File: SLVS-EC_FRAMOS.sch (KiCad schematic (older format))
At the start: 10 parts, among them J21 DF40HC(4.0)-60DS-0.4V(51)

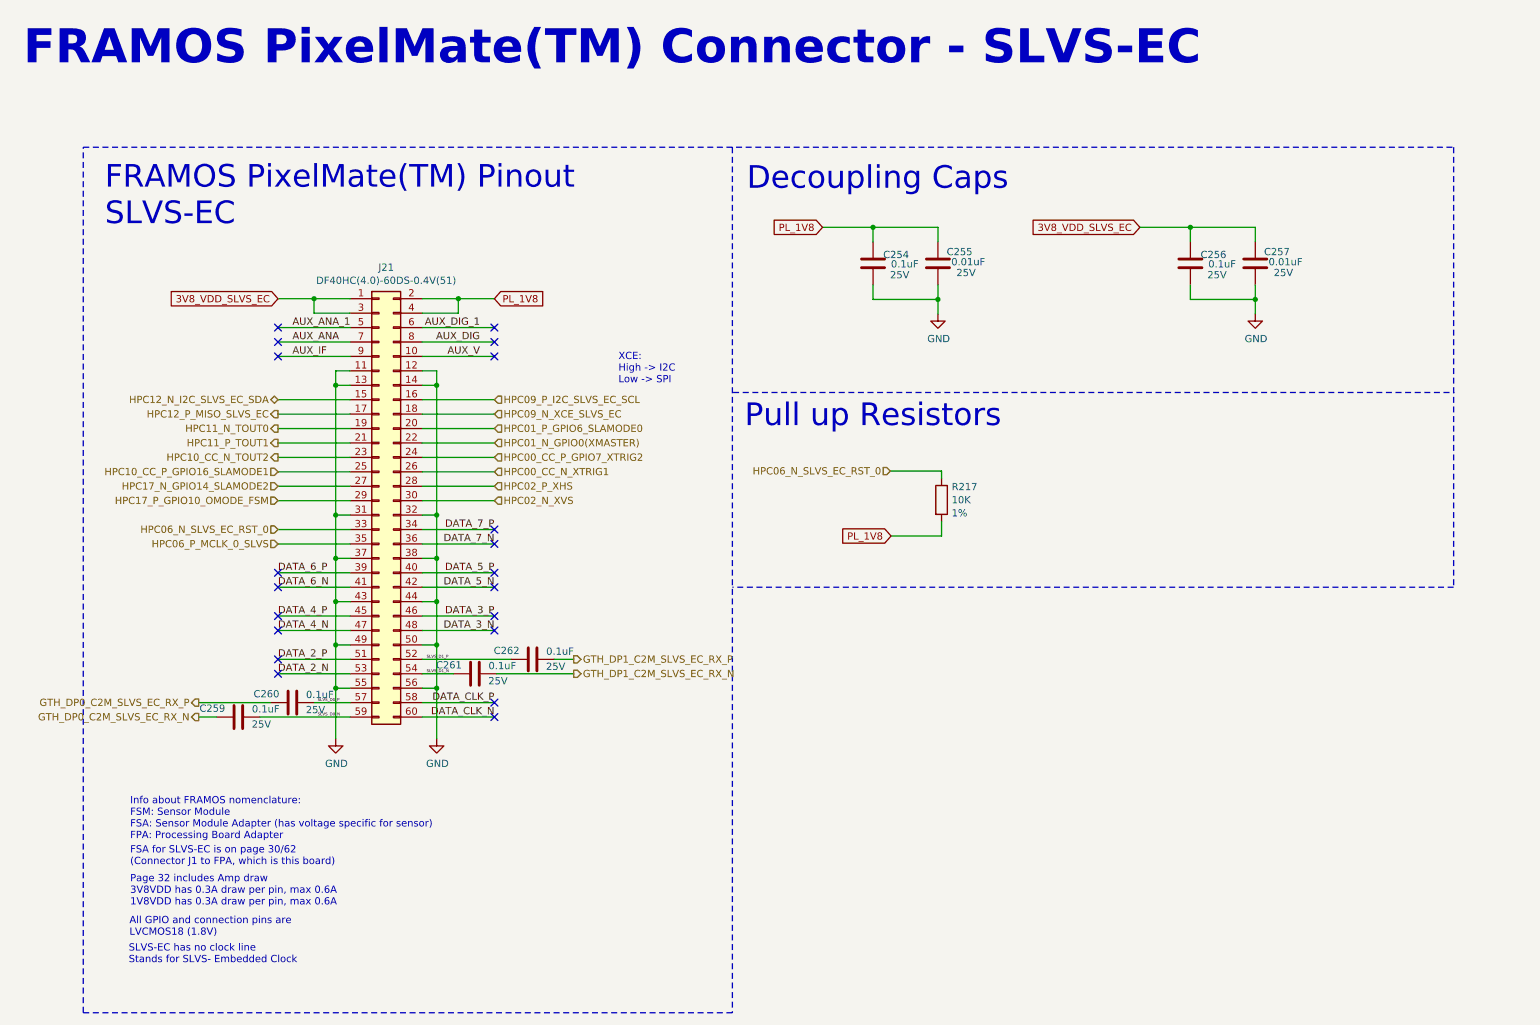
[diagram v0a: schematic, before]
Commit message: Pre-Production Push
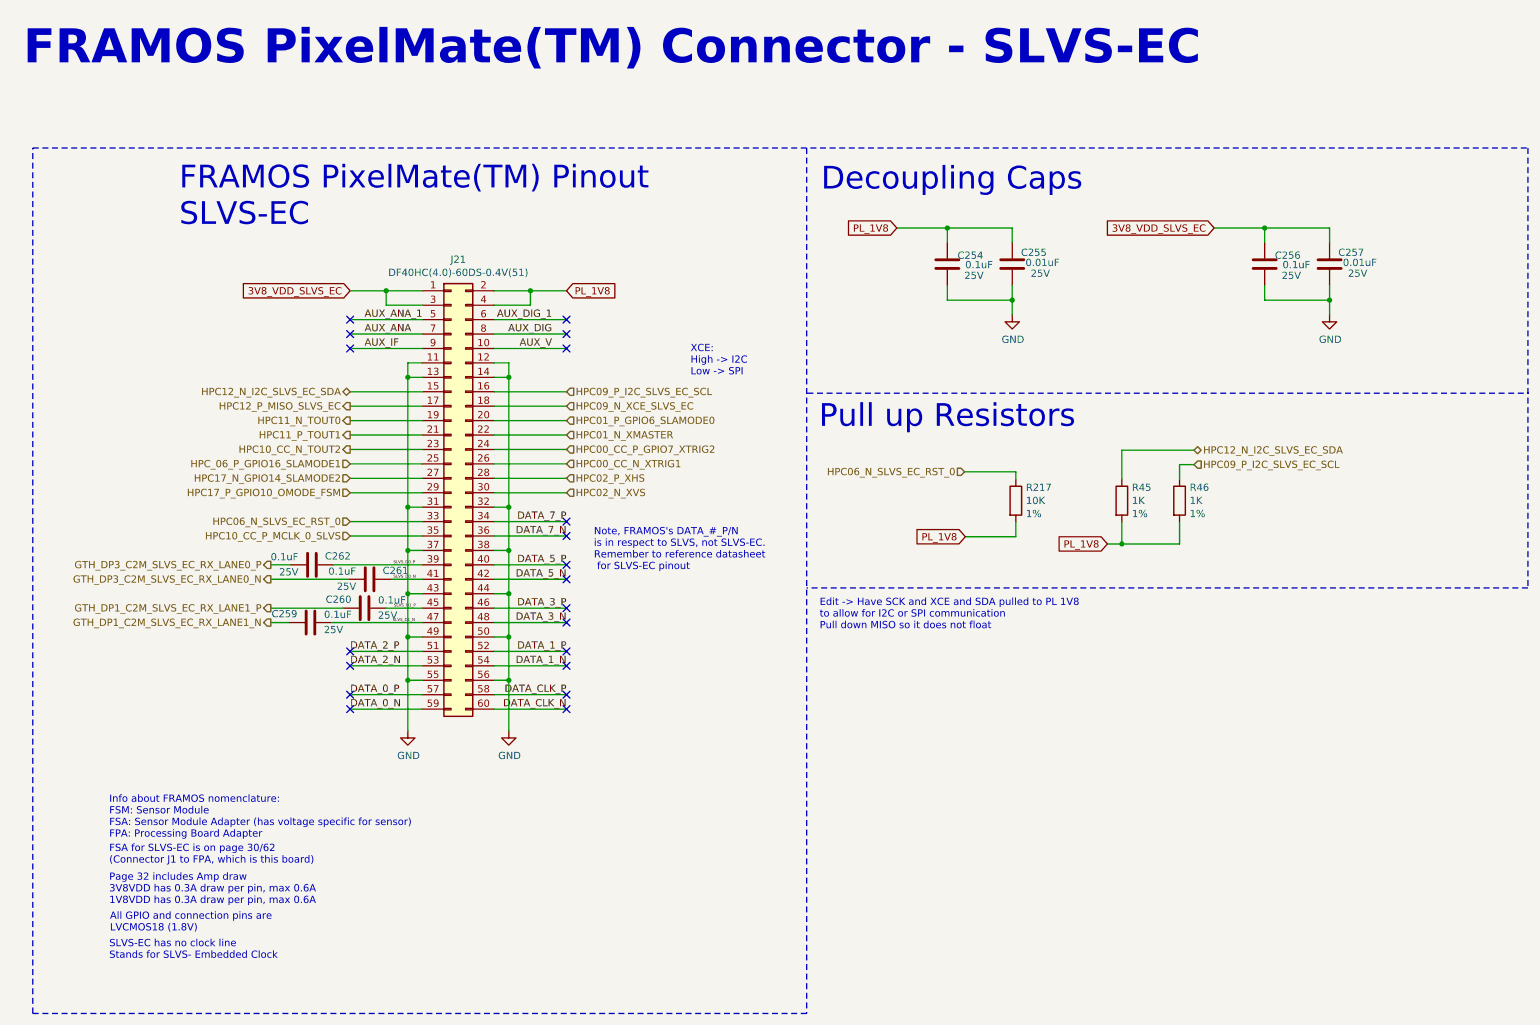
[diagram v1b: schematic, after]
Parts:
- added R45, R46: 1K, Resistor_SMD:R_0402_1005Metric, symbol Device:R
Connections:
- net DATA_4_N is gone; now on net SLVS_D1_N: J21.47 (Pin_47)
- net DATA_4_P is gone; now on net SLVS_D1_P: J21.45 (Pin_45)
- net DATA_6_N is gone; now on net SLVS_D0_N: J21.41 (Pin_41)
- net DATA_6_P is gone; now on net SLVS_D0_P: J21.39 (Pin_39)
- net HPC09_P_I2C_SLVS_EC_SCL: now also R46.1
- net HPC12_N_I2C_SLVS_EC_SDA: now also R45.1
- net PL_1V8: now also R45.2, R46.2
- net SLVS_D0_N: now also C261.2; no longer C259.1, J21.59 (Pin_59)
- net SLVS_D0_P: now also C262.2; no longer C260.1, J21.57 (Pin_57)
- net SLVS_D1_N: now also C259.1; no longer C261.2, J21.54 (Pin_54)
- net SLVS_D1_P: now also C260.1; no longer C262.2, J21.52 (Pin_52)
- net GTH_DP0_C2M_SLVS_EC_RX_N renamed GTH_DP1_C2M_SLVS_EC_RX_LANE1_N
- net GTH_DP0_C2M_SLVS_EC_RX_P renamed GTH_DP1_C2M_SLVS_EC_RX_LANE1_P
- net GTH_DP1_C2M_SLVS_EC_RX_N renamed GTH_DP3_C2M_SLVS_EC_RX_LANE0_N
- net GTH_DP1_C2M_SLVS_EC_RX_P renamed GTH_DP3_C2M_SLVS_EC_RX_LANE0_P
- net HPC01_N_GPIO0(XMASTER) renamed HPC01_N_XMASTER
- net HPC06_P_MCLK_0_SLVS renamed HPC10_CC_P_MCLK_0_SLVS
- net HPC10_CC_P_GPIO16_SLAMODE1 renamed HPC_06_P_GPIO16_SLAMODE1
- new net DATA_0_N: J21.59 (Pin_59)
- new net DATA_0_P: J21.57 (Pin_57)
- new net DATA_1_N: J21.54 (Pin_54)
- new net DATA_1_P: J21.52 (Pin_52)
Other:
- note added: "Edit -> Have SCK and XCE and SDA pulled to PL 1V8\nto allow for I2C or SPI communication\nPull down MISO so it does not float"
- note added: "Note, FRAMOS's DATA_#_P/N \nis in respect to SLVS, not SLVS-EC.\nRemember to reference datasheet\n for SLVS-EC pinout"
- moved on the sheet: C254, C255, C256, C257, C259, C260, C261, C262, J21, R217
